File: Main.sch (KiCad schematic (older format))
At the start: 60 parts, among them J1 Conn_01x01_Male, J2 Conn_01x06_Male, J3 Conn_01x05_Male, J4 Conn_01x01_Male, J5 Conn_01x05_Male, J6 Conn_01x03, J7 Conn_01x03, J8 Conn_01x06, J9 Conn_01x06_Male, Q1 CSD17307Q5A, Q2 CSD17307Q5A, U1 LM4120-CustomSymbols, U2 LTC2942, U3 LM393, U4 TPS2557, U5 LM393, U6 TPS2557, U7 SN74LVC2G08

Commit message: removed_switches
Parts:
- removed OUT1, SHORT1: SW_Push, Button_Switch_SMD:SW_DIP_SPSTx01_Slide_6.7x4.1mm_W6.73mm_P2.54mm_LowProfile_JPin, symbol Switch:SW_Push
- added JP1, JP2: Jumper_2_Open, Connector_PinHeader_2.00mm:PinHeader_1x02_P2.00mm_Vertical, symbol Jumper:Jumper_2_Open
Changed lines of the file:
@@
 Wire Wire Line
 	8900 7750 8700 7750
-$Comp
-L Switch:SW_Push OUT1
-U 1 1 5E2FB6C9
-P 9100 7750
-F 0 "OUT1" H 9000 8100 50  0000 L CNN
-F 1 "SW_Push" H 9000 8000 50  0000 L CNN
-F 2 "Button_Switch_SMD:SW_DIP_SPSTx01_Slide_6.7x4.1mm_W6.73mm_P2.54mm_LowProfile_JPin" H 9100 7950 50  0001 C CNN
-F 3 "~" H 9100 7950 50  0001 C CNN
-	1    9100 7750
-	1    0    0    -1
-$EndComp
 Wire Wire Line
 	7850 7750 8700 7750
@@
 Wire Wire Line
 	5800 8100 5800 7750
-$Comp
-L Switch:SW_Push SHORT1
-U 1 1 5D0F6604
-P 5800 8300
-F 0 "SHORT1" V 5754 8448 50  0000 L CNN
-F 1 "SW_Push" V 5845 8448 50  0000 L CNN
-F 2 "Button_Switch_SMD:SW_DIP_SPSTx01_Slide_6.7x4.1mm_W6.73mm_P2.54mm_LowProfile_JPin" H 5800 8500 50  0001 C CNN
-F 3 "~" H 5800 8500 50  0001 C CNN
-	1    5800 8300
-	0    1    1    0
-$EndComp
 Wire Wire Line
 	3150 8300 3150 8400
@@
 Wire Notes Line
 	1000 5000 1000 1100
+$Comp
+L Jumper:Jumper_2_Open JP2
+U 1 1 5DF47769
+P 9100 7750
+F 0 "JP2" H 9100 7525 50  0000 C CNN
+F 1 "Jumper_2_Open" H 9100 7600 50  0000 C CNN
+F 2 "Connector_PinHeader_2.00mm:PinHeader_1x02_P2.00mm_Vertical" H 9100 7750 50  0001 C CNN
+F 3 "~" H 9100 7750 50  0001 C CNN
+	1    9100 7750
+	1    0    0    -1
+$EndComp
+$Comp
+L Jumper:Jumper_2_Open JP1
+U 1 1 5DF5F15C
+P 5800 8300
+F 0 "JP1" H 5800 8075 50  0000 C CNN
+F 1 "Jumper_2_Open" H 5800 8150 50  0000 C CNN
+F 2 "Connector_PinHeader_2.00mm:PinHeader_1x02_P2.00mm_Vertical" H 5800 8300 50  0001 C CNN
+F 3 "~" H 5800 8300 50  0001 C CNN
+	1    5800 8300
+	0    -1   -1   0
+$EndComp
 $EndSCHEMATC

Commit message: progress
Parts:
- JP1, JP2: footprint Connector_PinHeader_2.00mm:PinHeader_1x02_P2.00mm_Vertical -> Connector_PinSocket_2.54mm:PinSocket_1x01_P2.54mm_Vertical
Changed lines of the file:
@@
 F 0 "JP2" H 9100 7525 50  0000 C CNN
 F 1 "Jumper_2_Open" H 9100 7600 50  0000 C CNN
-F 2 "Connector_PinHeader_2.00mm:PinHeader_1x02_P2.00mm_Vertical" H 9100 7750 50  0001 C CNN
+F 2 "Connector_PinSocket_2.54mm:PinSocket_1x01_P2.54mm_Vertical" H 9100 7750 50  0001 C CNN
 F 3 "~" H 9100 7750 50  0001 C CNN
 	1    9100 7750
@@
 F 0 "JP1" H 5800 8075 50  0000 C CNN
 F 1 "Jumper_2_Open" H 5800 8150 50  0000 C CNN
-F 2 "Connector_PinHeader_2.00mm:PinHeader_1x02_P2.00mm_Vertical" H 5800 8300 50  0001 C CNN
+F 2 "Connector_PinSocket_2.54mm:PinSocket_1x01_P2.54mm_Vertical" H 5800 8300 50  0001 C CNN
 F 3 "~" H 5800 8300 50  0001 C CNN
 	1    5800 8300

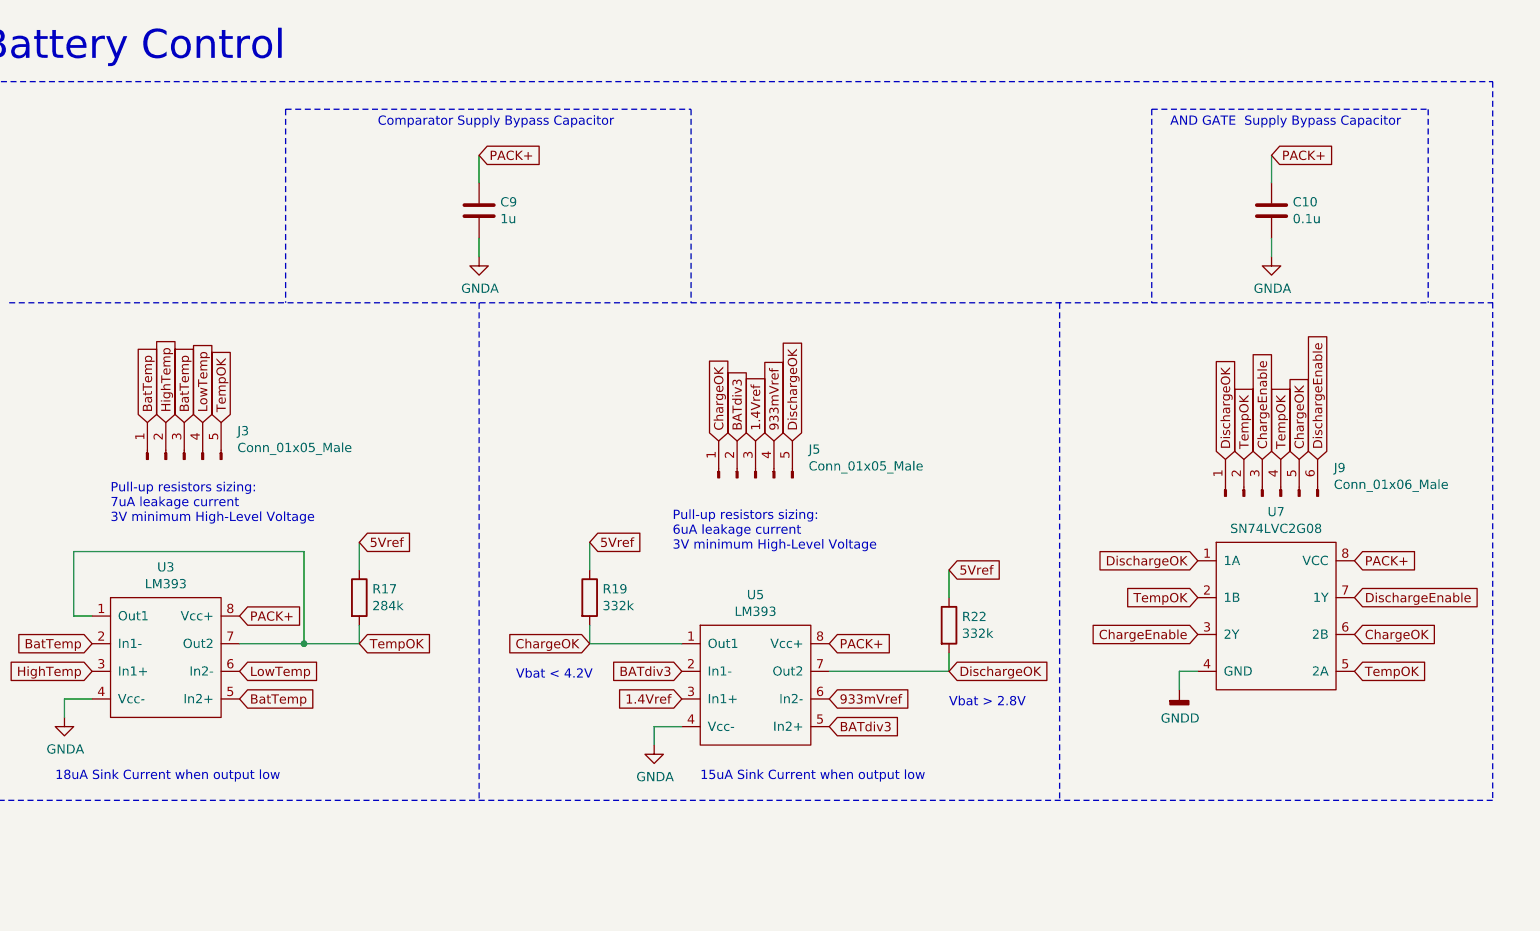
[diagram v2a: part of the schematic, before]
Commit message: progress
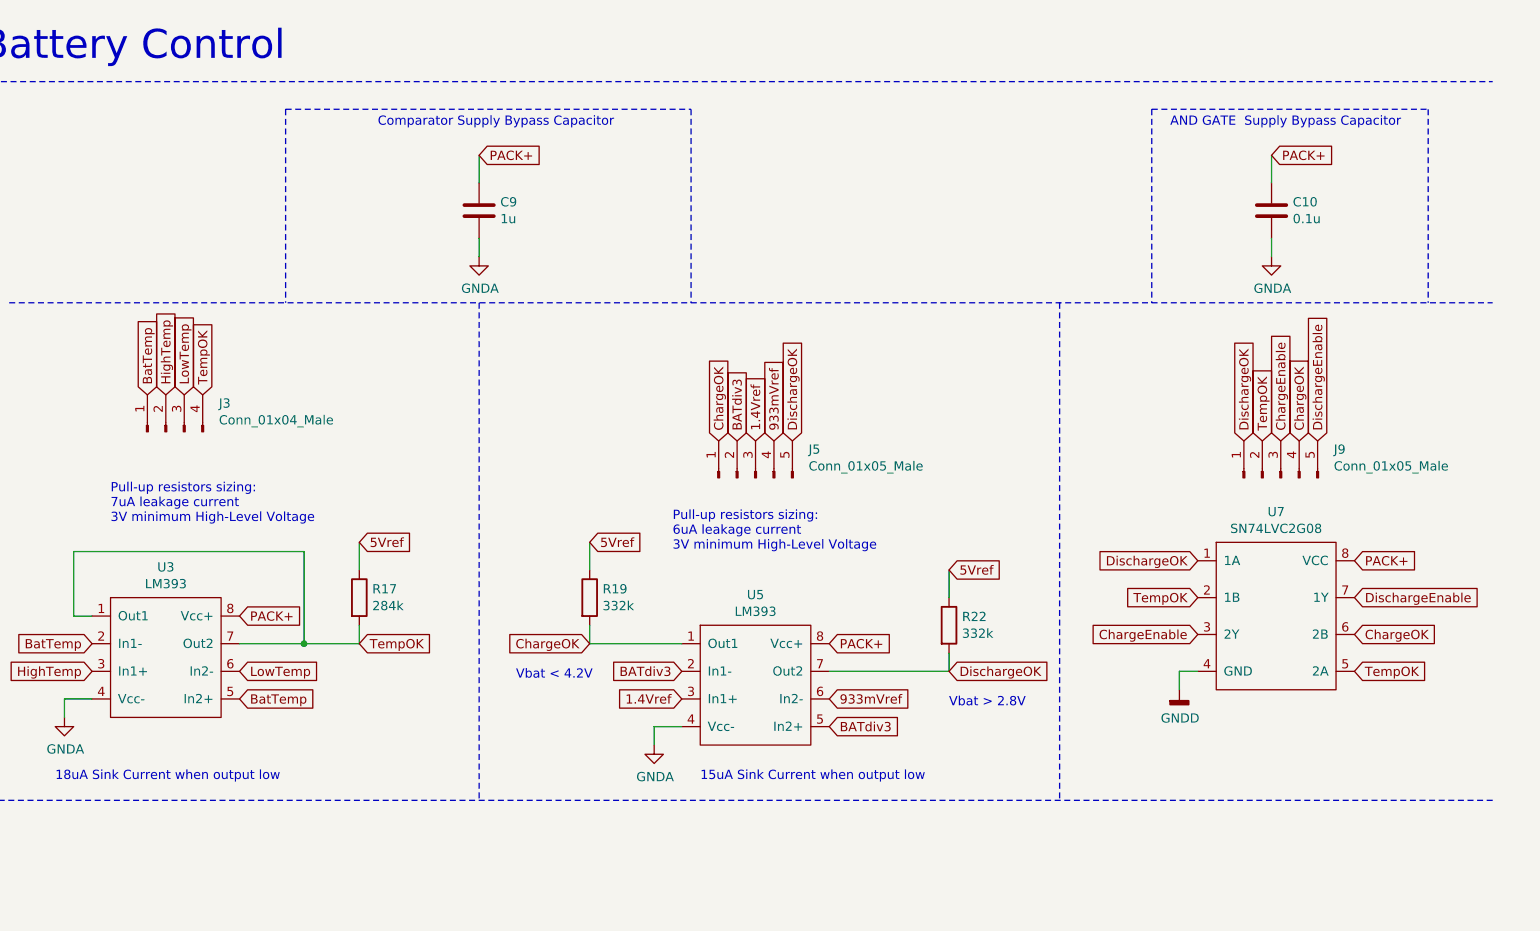
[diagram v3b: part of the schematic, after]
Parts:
- removed J3: Conn_01x05_Male, Connector_PinHeader_2.00mm:PinHeader_1x05_P2.00mm_Vertical, symbol Connector:Conn_01x05_Male
- removed J9: Conn_01x06_Male, Connector_PinHeader_2.00mm:PinHeader_1x06_P2.00mm_Vertical, symbol Connector:Conn_01x06_Male
- added J3: Conn_01x04_Male, Connector_PinHeader_2.00mm:PinHeader_1x04_P2.00mm_Vertical, symbol Connector:Conn_01x04_Male
- added J9: Conn_01x05_Male, Connector_PinHeader_2.00mm:PinHeader_1x05_P2.00mm_Vertical, symbol Connector:Conn_01x05_Male
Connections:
- net BatTemp: now also J3.1 (Pin_1)
- net ChargeEnable: now also J9.3 (Pin_3)
- net ChargeOK: now also J9.4 (Pin_4)
- net DischargeEnable: now also J9.5 (Pin_5)
- net DischargeOK: now also J9.1 (Pin_1)
- net HighTemp: now also J3.2 (Pin_2)
- net LowTemp: now also J3.3 (Pin_3)
- net TempOK: now also J3.4 (Pin_4), J9.2 (Pin_2)
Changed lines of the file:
@@
 	0    -1   -1   0
 $EndComp
-$Comp
-L Connector:Conn_01x05_Male J3
-U 1 1 5DFA2C02
-P 8350 3150
-F 0 "J3" V 8504 2862 50  0000 R CNN
-F 1 "Conn_01x05_Male" V 8413 2862 50  0000 R CNN
-F 2 "Connector_PinHeader_2.00mm:PinHeader_1x05_P2.00mm_Vertical" H 8350 3150 50  0001 C CNN
-F 3 "~" H 8350 3150 50  0001 C CNN
-	1    8350 3150
-	0    -1   -1   0
-$EndComp
-Text GLabel 8150 2950 1    50   Input ~ 0
+Text GLabel 8150 2800 1    50   Input ~ 0
 BatTemp
-Text GLabel 8250 2950 1    50   Input ~ 0
+Text GLabel 8250 2800 1    50   Input ~ 0
 HighTemp
-Text GLabel 8350 2950 1    50   Input ~ 0
-BatTemp
-Text GLabel 8450 2950 1    50   Input ~ 0
+Text GLabel 8350 2800 1    50   Input ~ 0
 LowTemp
-Text GLabel 8550 2950 1    50   Input ~ 0
+Text GLabel 8450 2800 1    50   Input ~ 0
 TempOK
-Text GLabel 14300 3150 1    50   Input ~ 0
+Text GLabel 14400 3050 1    50   Input ~ 0
+ChargeOK
+Text GLabel 14500 3050 1    50   Input ~ 0
+DischargeEnable
+Text GLabel 14300 3050 1    50   Input ~ 0
+ChargeEnable
+Text GLabel 14200 3050 1    50   Input ~ 0
 TempOK
-Text GLabel 14400 3150 1    50   Input ~ 0
-ChargeOK
-Text GLabel 14500 3150 1    50   Input ~ 0
-DischargeEnable
-Text GLabel 14200 3150 1    50   Input ~ 0
-ChargeEnable
-Text GLabel 14100 3150 1    50   Input ~ 0
-TempOK
-Text GLabel 14000 3150 1    50   Input ~ 0
+Text GLabel 14100 3050 1    50   Input ~ 0
 DischargeOK
-$Comp
-L Connector:Conn_01x06_Male J9
-U 1 1 5DFC1AB1
-P 14200 3350
-F 0 "J9" V 14354 2962 50  0000 R CNN
-F 1 "Conn_01x06_Male" V 14263 2962 50  0000 R CNN
-F 2 "Connector_PinHeader_2.00mm:PinHeader_1x06_P2.00mm_Vertical" H 14200 3350 50  0001 C CNN
-F 3 "~" H 14200 3350 50  0001 C CNN
-	1    14200 3350
-	0    -1   -1   0
-$EndComp
 $Comp
 L Main-rescue:SN74LVC2G08-CustomSymbols U7
@@
 Wire Notes Line
 	1000 1100 15450 1100
-Wire Notes Line
-	15450 1100 15450 5000
 Text Notes 7250 1000 0    157  ~ 0
 Battery Control
@@
 	0    -1   -1   0
 $EndComp
+$Comp
+L Connector:Conn_01x04_Male J3
+U 1 1 5DF9ED68
+P 8250 3000
+F 0 "J3" V 8404 2712 50  0000 R CNN
+F 1 "Conn_01x04_Male" V 8313 2712 50  0000 R CNN
+F 2 "Connector_PinHeader_2.00mm:PinHeader_1x04_P2.00mm_Vertical" H 8250 3000 50  0001 C CNN
+F 3 "~" H 8250 3000 50  0001 C CNN
+	1    8250 3000
+	0    -1   -1   0
+$EndComp
+$Comp
+L Connector:Conn_01x05_Male J9
+U 1 1 5E03D4C2
+P 14300 3250
+F 0 "J9" V 14454 2962 50  0000 R CNN
+F 1 "Conn_01x05_Male" V 14363 2962 50  0000 R CNN
+F 2 "Connector_PinHeader_2.00mm:PinHeader_1x05_P2.00mm_Vertical" H 14300 3250 50  0001 C CNN
+F 3 "~" H 14300 3250 50  0001 C CNN
+	1    14300 3250
+	0    -1   -1   0
+$EndComp
